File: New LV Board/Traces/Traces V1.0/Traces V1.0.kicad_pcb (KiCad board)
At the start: 2 copper layers, 126.6 x 49.2 mm, 13 parts, among them J1 B15B-PH-K-S, J2 B15B-PH-K-S, J3 B15B-PH-K-S, J4 Conn_01x12, J6 Conn_01x12, J7 Conn_01x12

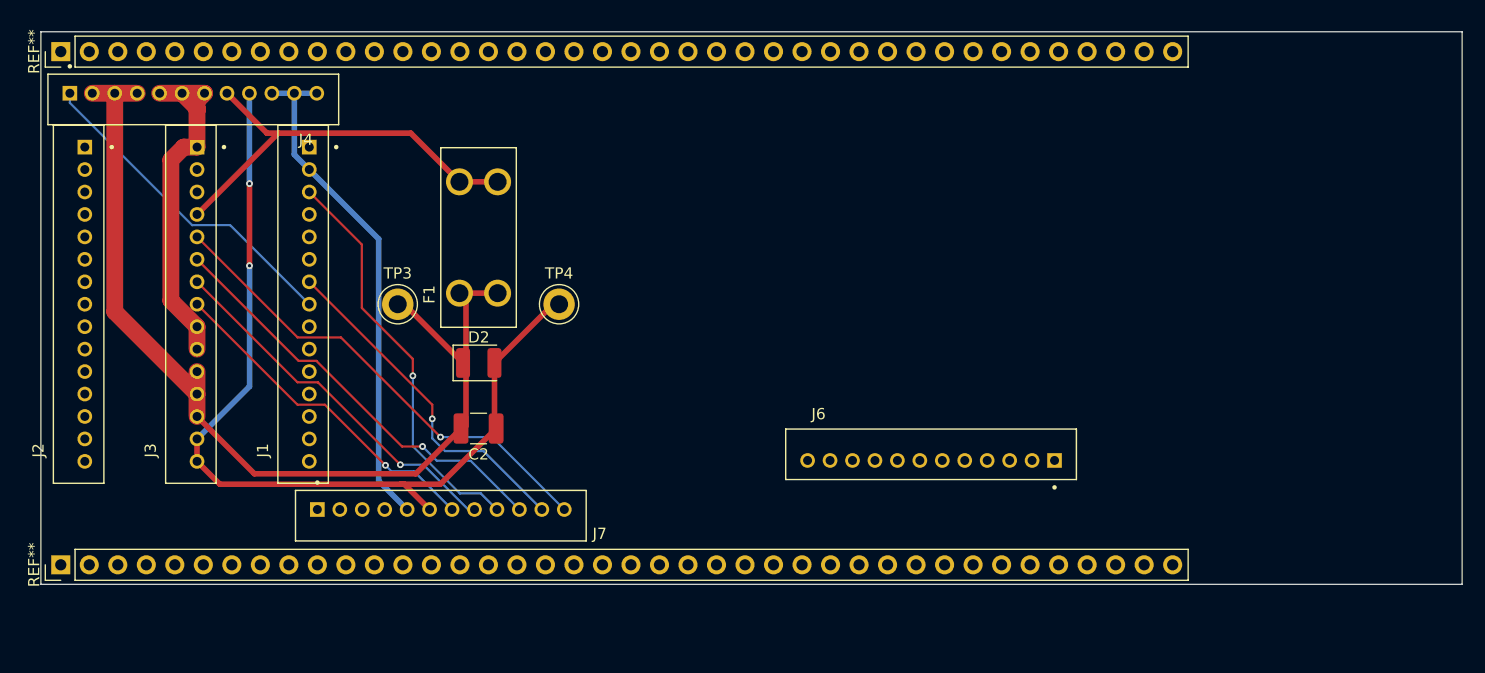
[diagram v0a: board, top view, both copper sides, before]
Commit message: TRACES IS DONE
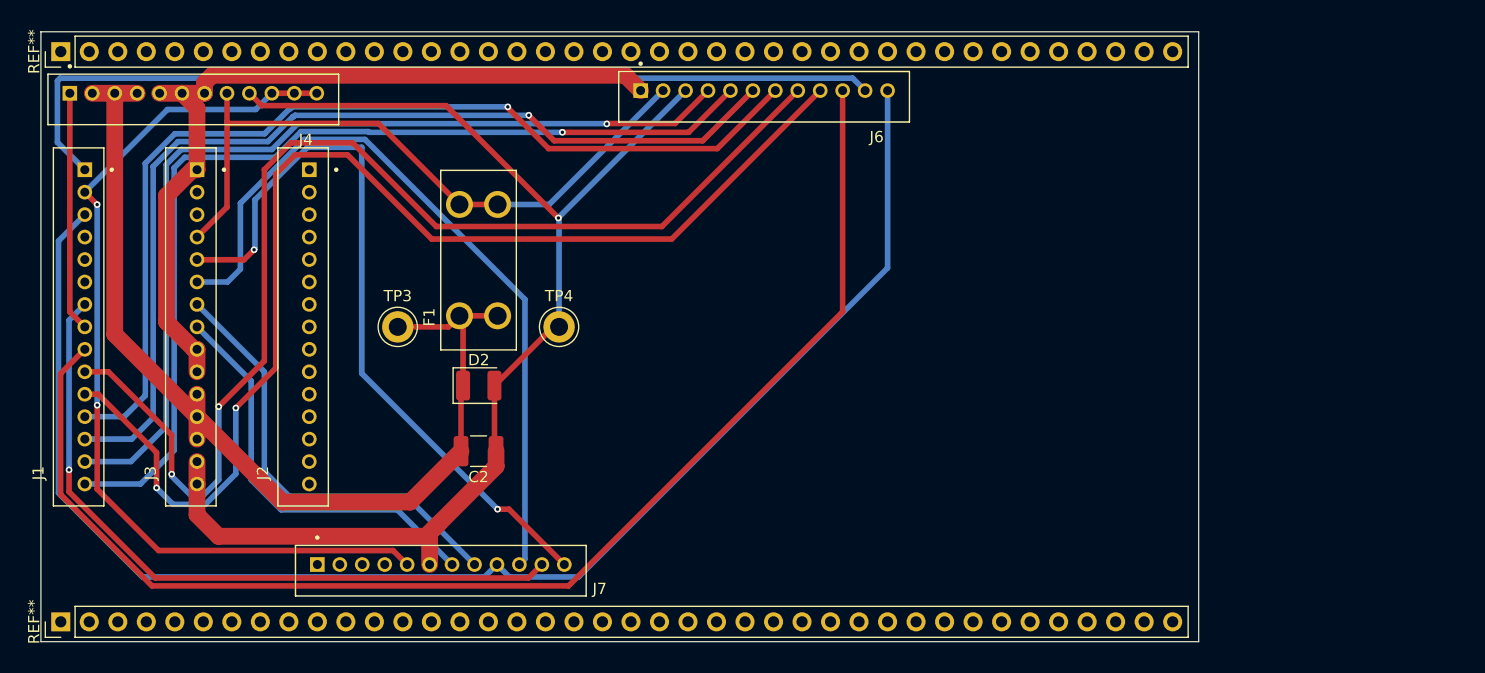
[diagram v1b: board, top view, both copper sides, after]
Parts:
- moved J6 35.2 mm to (108.4, 100.8), turned to 180 degrees
- moved J1 20.1 mm to (47.3, 121.3)
- moved J2 20.1 mm to (67.3, 121.3)
- moved REF** 5.08 mm to (45.7, 147.6)
- moved J7 4.90 mm to (79.6, 143.0)
- moved D2 2.02 mm to (83.0, 126.5)
- moved F1 2.02 mm to (82.9, 115.4)
- moved C2 2.02 mm to (82.9, 132.4)
- moved J3 2.02 mm to (57.3, 121.3)
- moved TP3 2.02 mm to (75.7, 121.3)
- moved TP4 2.02 mm to (90.1, 121.3)
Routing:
- net Net-(J6-Pin_10): track 0.00 -> 116.7 mm
- net Net-(J6-Pin_9): track 0.00 -> 106.5 mm, vias 0 -> 2
- net Net-(J6-Pin_8): track 0.00 -> 105.3 mm, vias 0 -> 2
- net Net-(J6-Pin_12): track 36.3 -> 130.9 mm, vias 1 -> 0
- net Net-(J6-Pin_7): track 0.00 -> 88.8 mm, vias 0 -> 1
- net Net-(J6-Pin_6): track 0.00 -> 87.4 mm, vias 0 -> 1
- net Net-(J6-Pin_5): track 0.00 -> 86.8 mm, vias 0 -> 1
- net Net-(J6-Pin_4): track 0.00 -> 82.9 mm, vias 0 -> 1
- net Net-(J6-Pin_11): track 0.00 -> 81.4 mm
- net Net-(J4-Pin_5): track 31.8 -> 72.6 mm
- net Net-(J4-Pin_10): track 45.2 -> 81.6 mm, vias 0 -> 2
- net Net-(J7-Pin_11): track 30.9 -> 63.1 mm
- net Net-(D2-A): track 81.6 -> 111.8 mm, vias 2 -> 1
- net Net-(J7-Pin_10): track 38.0 -> 67.6 mm, vias 1 -> 0
- net Net-(J7-Pin_12): track 43.0 -> 66.6 mm, vias 1 -> 2
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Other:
- board size 126.6 x 49.2 mm -> 103.1 x 54.3 mm
